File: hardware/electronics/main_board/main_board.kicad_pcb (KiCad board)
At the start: 2 copper layers, 5 parts

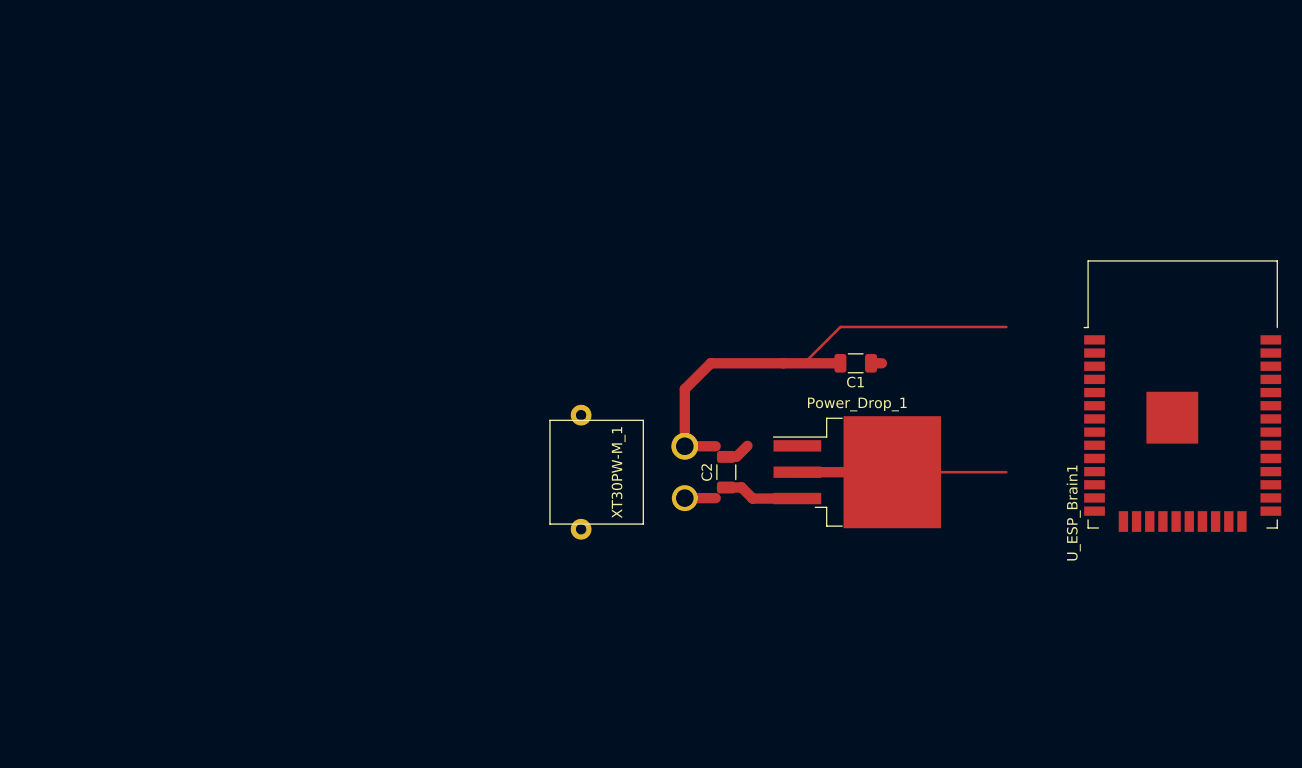
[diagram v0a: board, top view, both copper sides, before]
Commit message: pcb looking much better
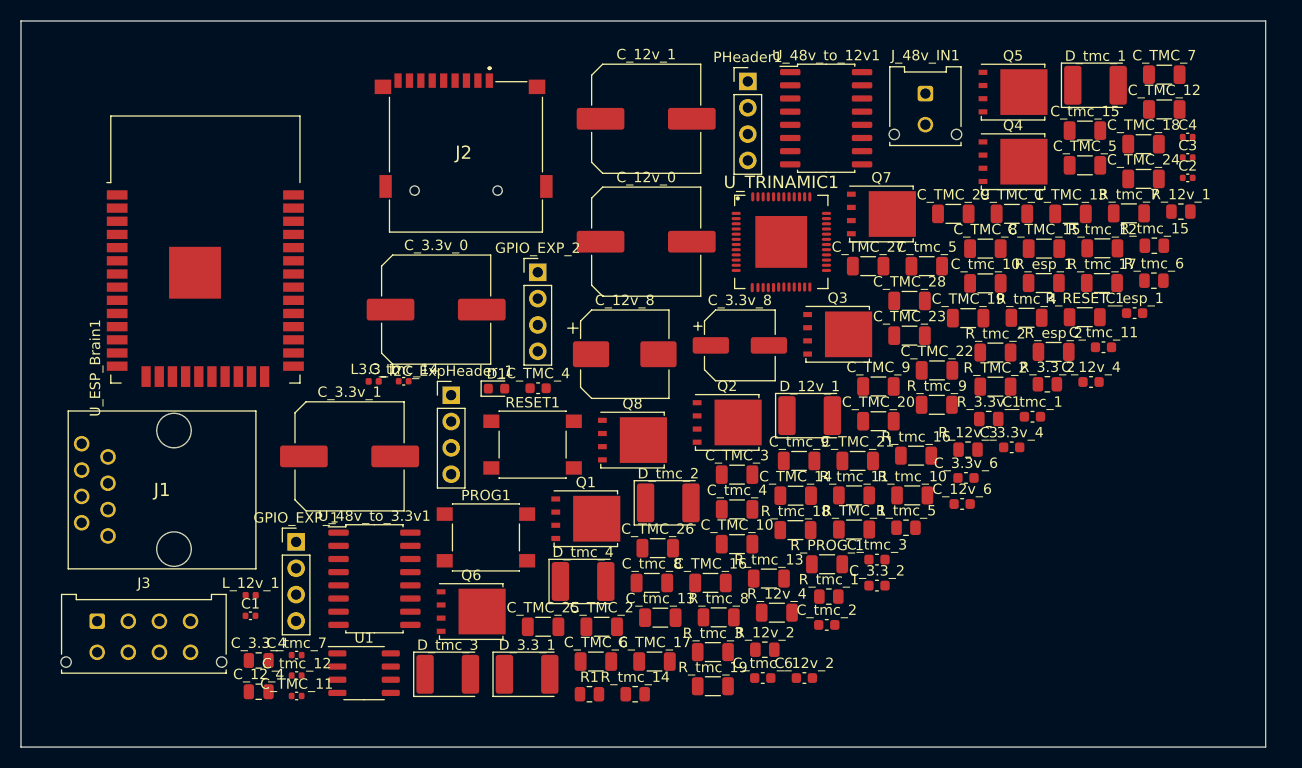
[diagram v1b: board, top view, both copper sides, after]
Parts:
- removed Power_Drop_1: LM1085-3.3, Package_TO_SOT_SMD:TO-263-3_TabPin2
- removed XT30PW-M_1: 24v DC In, main_board:XT30PW-M
- added C3: 10uF, Capacitor_SMD:C_0402_1005Metric, F.Cu at (172.5, 53.2)
- added C4: 100nF, Capacitor_SMD:C_0402_1005Metric, F.Cu at (172.5, 51.2)
- added C_12_4: 22nF, Capacitor_SMD:C_0805_2012Metric, F.Cu at (82.9, 104.7)
- added C_12v_0: 220uF, Capacitor_SMD:C_Elec_10x10.2, F.Cu at (120.3, 61.3)
- added C_12v_1: 220uF, Capacitor_SMD:C_Elec_10x10.2, F.Cu at (120.3, 49.4)
- added C_12v_2: 2.7nF, Capacitor_SMD:C_0603_1608Metric, F.Cu at (135.5, 103.3)
- added C_12v_4: 100nF, Capacitor_SMD:C_0603_1608Metric, F.Cu at (163.2, 74.8)
- added C_12v_6: 100nF, Capacitor_SMD:C_0603_1608Metric, F.Cu at (150.7, 86.6)
- added C_12v_8: 330uF, Capacitor_SMD:CP_Elec_8x10, F.Cu at (118.2, 72.1)
- added C_3.3_2: 2.7nF, Capacitor_SMD:C_0603_1608Metric, F.Cu at (142.5, 94.4)
- added C_3.3_4: 22nF, Capacitor_SMD:C_0805_2012Metric, F.Cu at (82.9, 101.7)
- added C_3.3v_0: 220uF, Capacitor_SMD:C_Elec_10x10.2, F.Cu at (100.0, 67.8)
- added C_3.3v_1: 220uF, Capacitor_SMD:C_Elec_10x10.2, F.Cu at (91.7, 82.0)
- added C_3.3v_4: 100nF, Capacitor_SMD:C_0603_1608Metric, F.Cu at (155.5, 81.1)
- added C_3.3v_6: 100nF, Capacitor_SMD:C_0603_1608Metric, F.Cu at (151.1, 84.1)
- added C_3.3v_8: 330uF, Capacitor_SMD:CP_Elec_6.3x5.9, F.Cu at (129.3, 71.3)
- added C_TMC_1: 1n, Capacitor_SMD:C_1206_3216Metric, F.Cu at (155.5, 58.6)
- added C_TMC_10: 1n, Capacitor_SMD:C_1206_3216Metric, F.Cu at (129.0, 90.4)
- added C_TMC_11: 100n, Capacitor_SMD:C_0402_1005Metric, F.Cu at (86.6, 105.1)
- added C_TMC_12: 1n, Capacitor_SMD:C_1206_3216Metric, F.Cu at (170.2, 48.5)
- added C_TMC_13: 1n, Capacitor_SMD:C_1206_3216Metric, F.Cu at (161.2, 58.6)
- added C_TMC_14: 100nF, Capacitor_SMD:C_1206_3216Metric, F.Cu at (134.7, 85.8)
- added C_TMC_15: 1n, Capacitor_SMD:C_1206_3216Metric, F.Cu at (158.6, 61.9)
- added C_TMC_16: 1n, Capacitor_SMD:C_1206_3216Metric, F.Cu at (126.5, 94.2)
- added C_TMC_17: 1n, Capacitor_SMD:C_1206_3216Metric, F.Cu at (121.1, 101.8)
- added C_TMC_18: 1n, Capacitor_SMD:C_1206_3216Metric, F.Cu at (168.2, 51.9)
- added C_TMC_19: 1n, Capacitor_SMD:C_1206_3216Metric, F.Cu at (151.3, 68.6)
- added C_TMC_2: 1n, Capacitor_SMD:C_1206_3216Metric, F.Cu at (116.0, 98.4)
- added C_TMC_20: 1n, Capacitor_SMD:C_1206_3216Metric, F.Cu at (142.7, 78.6)
- added C_TMC_21: 1n, Capacitor_SMD:C_1206_3216Metric, F.Cu at (140.7, 82.4)
- added C_TMC_22: 1n, Capacitor_SMD:C_1206_3216Metric, F.Cu at (148.3, 73.7)
- added C_TMC_23: 1n, Capacitor_SMD:C_1206_3216Metric, F.Cu at (145.7, 70.3)
- added C_TMC_24: 1n, Capacitor_SMD:C_1206_3216Metric, F.Cu at (168.2, 55.2)
- added C_TMC_25: 1n, Capacitor_SMD:C_1206_3216Metric, F.Cu at (110.3, 98.4)
- added C_TMC_26: 1n, Capacitor_SMD:C_1206_3216Metric, F.Cu at (121.4, 90.8)
- added C_TMC_27: 1n, Capacitor_SMD:C_1206_3216Metric, F.Cu at (141.7, 63.6)
- added C_TMC_28: 1n, Capacitor_SMD:C_1206_3216Metric, F.Cu at (145.7, 67.0)
- added C_TMC_29: 1n, Capacitor_SMD:C_1206_3216Metric, F.Cu at (149.9, 58.6)
- added C_TMC_3: 1n, Capacitor_SMD:C_1206_3216Metric, F.Cu at (129.0, 83.7)
- added C_TMC_4: 100nF, Capacitor_SMD:C_0603_1608Metric, F.Cu at (109.9, 75.4)
- added C_TMC_5: 1n, Capacitor_SMD:C_1206_3216Metric, F.Cu at (162.6, 53.9)
- added C_TMC_6: 1n, Capacitor_SMD:C_1206_3216Metric, F.Cu at (115.4, 101.8)
- added C_TMC_7: 1n, Capacitor_SMD:C_1206_3216Metric, F.Cu at (170.2, 45.2)
- added C_TMC_8: 1n, Capacitor_SMD:C_1206_3216Metric, F.Cu at (153.0, 61.9)
- added C_TMC_9: 1n, Capacitor_SMD:C_1206_3216Metric, F.Cu at (142.7, 75.2)
- added C_esp_1: 470n, Capacitor_SMD:C_0603_1608Metric, F.Cu at (167.4, 68.2)
- added C_tmc_1: 2.2u, Capacitor_SMD:C_0603_1608Metric, F.Cu at (157.5, 78.2)
- added C_tmc_10: 220nF, Capacitor_SMD:C_1206_3216Metric, F.Cu at (153.0, 65.3)
- added C_tmc_11: 2.2u, Capacitor_SMD:C_0603_1608Metric, F.Cu at (164.4, 71.5)
- added C_tmc_12: 100nF, Capacitor_SMD:C_0402_1005Metric, F.Cu at (86.6, 103.1)
- added C_tmc_13: 4.7uF, Capacitor_SMD:C_1206_3216Metric, F.Cu at (121.6, 97.5)
- added C_tmc_14: 100nF, Capacitor_SMD:C_0402_1005Metric, F.Cu at (96.9, 74.7)
- added C_tmc_15: 4.7uF, Capacitor_SMD:C_1206_3216Metric, F.Cu at (162.6, 50.6)
- added C_tmc_2: 2.2u, Capacitor_SMD:C_0603_1608Metric, F.Cu at (137.7, 98.2)
- added C_tmc_3: 470n, Capacitor_SMD:C_0603_1608Metric, F.Cu at (142.5, 91.9)
- added C_tmc_4: 220nF, Capacitor_SMD:C_1206_3216Metric, F.Cu at (129.0, 87.1)
- added C_tmc_5: 220nF, Capacitor_SMD:C_1206_3216Metric, F.Cu at (147.3, 63.6)
- added C_tmc_6: 2.2u, Capacitor_SMD:C_0603_1608Metric, F.Cu at (131.5, 103.3)
- added C_tmc_7: 100nF, Capacitor_SMD:C_0402_1005Metric, F.Cu at (86.6, 101.1)
- added C_tmc_8: 470nF, Capacitor_SMD:C_1206_3216Metric, F.Cu at (120.8, 94.2)
- added C_tmc_9: 220nF, Capacitor_SMD:C_1206_3216Metric, F.Cu at (135.0, 82.4)
- added D1: LED, LED_SMD:LED_0603_1608Metric, F.Cu at (105.8, 75.4)
- added D_12v_1: STPS3L60U, Diode_SMD:D_2114_3652Metric, F.Cu at (136.0, 78.0)
- added D_3.3_1: STPS3L60U, Diode_SMD:D_2114_3652Metric, F.Cu at (108.8, 103.0)
- added D_tmc_1: STPS3L60U, Diode_SMD:D_2114_3652Metric, F.Cu at (163.6, 46.2)
- added D_tmc_2: STPS3L60U, Diode_SMD:D_2114_3652Metric, F.Cu at (122.4, 86.5)
- added D_tmc_3: STPS3L60U, Diode_SMD:D_2114_3652Metric, F.Cu at (101.1, 103.0)
- added D_tmc_4: STPS3L60U, Diode_SMD:D_2114_3652Metric, F.Cu at (114.2, 94.0)
- added GPIO_EXP_1: Conn_01x04_Male, Connector_PinHeader_2.54mm:PinHeader_1x04_P2.54mm_Vertical, F.Cu at (86.5, 90.2)
- added GPIO_EXP_2: Conn_01x04_Male, Connector_PinHeader_2.54mm:PinHeader_1x04_P2.54mm_Vertical, F.Cu at (109.8, 64.2)
- added I2C_ExpHeader_1: Conn_01x04_Male, Connector_PinHeader_2.54mm:PinHeader_1x04_P2.54mm_Vertical, F.Cu at (101.5, 76.1)
- added J1: 215877-1, main_board:2158771, F.Cu at (65.9, 80.8)
- added J2: TF-15X15, main_board:TF15X15, F.Cu at (102.7, 52.7)
- added J3: Conn_02x04_Odd_Even, Connector_Molex:Molex_Micro-Fit_3.0_43045-0812_2x04_P3.00mm_Vertical, F.Cu at (67.3, 97.9)
- added J_48v_IN1: Molex, Connector_Molex:Molex_Micro-Fit_3.0_43045-0212_2x01_P3.00mm_Vertical, F.Cu at (147.2, 47.0)
- added L3.3_1: 126uH, Inductor_SMD:L_0402_1005Metric, F.Cu at (94.0, 74.7)
- added L_12v_1: 126uH, Inductor_SMD:L_0402_1005Metric, F.Cu at (82.1, 95.4)
- added PHeader1: Conn_01x04_Male, Connector_PinHeader_2.54mm:PinHeader_1x04_P2.54mm_Vertical, F.Cu at (130.1, 45.8)
- added PROG1: SW_Push_Dual_x2, Button_Switch_SMD:SW_Push_1P1T_NO_6x6mm_H9.5mm, F.Cu at (104.8, 89.8)
- added Q1: CSD18537NQ5A, Package_TO_SOT_SMD:TDSON-8-1, F.Cu at (114.5, 88.0)
- added Q2: CSD18537NQ5A, Package_TO_SOT_SMD:TDSON-8-1, F.Cu at (128.1, 78.7)
- added Q3: CSD18537NQ5A, Package_TO_SOT_SMD:TDSON-8-1, F.Cu at (138.7, 70.2)
- added Q4: CSD18537NQ5A, Package_TO_SOT_SMD:TDSON-8-1, F.Cu at (155.6, 53.6)
- added Q5: CSD18537NQ5A, Package_TO_SOT_SMD:TDSON-8-1, F.Cu at (155.6, 46.9)
- added Q6: CSD18537NQ5A, Package_TO_SOT_SMD:TDSON-8-1, F.Cu at (103.4, 96.9)
- added Q7: CSD18537NQ5A, Package_TO_SOT_SMD:TDSON-8-1, F.Cu at (143.0, 58.6)
- added Q8: CSD18537NQ5A, Package_TO_SOT_SMD:TDSON-8-1, F.Cu at (119.0, 80.4)
- added R1: 300 Ohms, Resistor_SMD:R_0805_2012Metric, F.Cu at (114.8, 104.9)
- added RESET1: SW_Push_Dual_x2, Button_Switch_SMD:SW_Push_1P1T_NO_6x6mm_H9.5mm, F.Cu at (109.3, 80.8)
- added R_12v_1: 20Kohms, Resistor_SMD:R_0805_2012Metric, F.Cu at (171.8, 58.4)
- added R_12v_2: 9.1kohms, Resistor_SMD:R_0805_2012Metric, F.Cu at (131.7, 100.6)
- added R_12v_3: 12kOhms, Resistor_SMD:R_0805_2012Metric, F.Cu at (151.3, 81.3)
- added R_12v_4: 4.7KOhms, Resistor_SMD:R_1206_3216Metric, F.Cu at (132.9, 97.0)
- added R_3.3_2: 9.1kohms, Resistor_SMD:R_0805_2012Metric, F.Cu at (159.0, 75.0)
- added R_3.3v_1: 20Kohms, Resistor_SMD:R_0805_2012Metric, F.Cu at (153.3, 78.4)
- added R_PROG_1: 10kOhms, Resistor_SMD:R_1206_3216Metric, F.Cu at (137.7, 92.4)
- added R_RESET_1: 10kOhms, Resistor_SMD:R_1206_3216Metric, F.Cu at (162.6, 68.6)
- added R_TMC_1: 10kOhms, Resistor_SMD:R_1206_3216Metric, F.Cu at (140.3, 89.0)
- added R_TMC_2: 10kOhms, Resistor_SMD:R_1206_3216Metric, F.Cu at (153.9, 75.3)
- added R_esp_1: 4.7KOhms, Resistor_SMD:R_1206_3216Metric, F.Cu at (158.6, 65.3)
- added R_esp_2: 4.7KOhms, Resistor_SMD:R_1206_3216Metric, F.Cu at (159.6, 71.9)
- added R_tmc_1: 2R2, Resistor_SMD:R_0805_2012Metric, F.Cu at (137.9, 95.5)
- added R_tmc_10: 10Ohm, Resistor_SMD:R_1206_3216Metric, F.Cu at (145.9, 85.7)
- added R_tmc_11: 10Ohm, Resistor_SMD:R_1206_3216Metric, F.Cu at (140.3, 85.7)
- added R_tmc_12: 10Ohm, Resistor_SMD:R_1206_3216Metric, F.Cu at (164.3, 61.9)
- added R_tmc_13: 10Ohm, Resistor_SMD:R_1206_3216Metric, F.Cu at (132.1, 93.8)
- added R_tmc_14: 47R, Resistor_SMD:R_0805_2012Metric, F.Cu at (119.2, 104.9)
- added R_tmc_15: 47R, Resistor_SMD:R_0805_2012Metric, F.Cu at (169.3, 61.7)
- added R_tmc_16: 10Ohm, Resistor_SMD:R_1206_3216Metric, F.Cu at (146.3, 81.9)
- added R_tmc_17: 10Ohm, Resistor_SMD:R_1206_3216Metric, F.Cu at (164.2, 65.3)
- added R_tmc_18: 10Ohm, Resistor_SMD:R_1206_3216Metric, F.Cu at (134.7, 89.1)
- added R_tmc_19: 10Ohm, Resistor_SMD:R_1206_3216Metric, F.Cu at (126.7, 104.1)
- added R_tmc_2: 10Ohm, Resistor_SMD:R_1206_3216Metric, F.Cu at (153.9, 72.0)
- added R_tmc_3: 10Ohm, Resistor_SMD:R_1206_3216Metric, F.Cu at (126.7, 100.8)
- added R_tmc_4: 10Ohm, Resistor_SMD:R_1206_3216Metric, F.Cu at (156.9, 68.6)
- added R_tmc_5: 47R, Resistor_SMD:R_0805_2012Metric, F.Cu at (145.3, 88.9)
- added R_tmc_6: 47R, Resistor_SMD:R_0805_2012Metric, F.Cu at (169.2, 65.0)
- added R_tmc_7: 10Ohm, Resistor_SMD:R_1206_3216Metric, F.Cu at (166.8, 58.5)
- added R_tmc_8: 10Ohm, Resistor_SMD:R_1206_3216Metric, F.Cu at (127.3, 97.5)
- added R_tmc_9: 10Ohm, Resistor_SMD:R_1206_3216Metric, F.Cu at (148.3, 77.0)
- added U1: P82B96, Package_SO:SO-8_3.9x4.9mm_P1.27mm, F.Cu at (93.1, 102.9)
- added U_48v_to_12v1: L4978D, Package_SO:SO-16_5.3x10.2mm_P1.27mm, F.Cu at (137.6, 49.4)
- added U_48v_to_3.3v1: L4978D, Package_SO:SO-16_5.3x10.2mm_P1.27mm, F.Cu at (94.1, 93.8)
- added U_TRINAMIC1: TMC5160-TA, trinamic-footprints:eTQFP48, F.Cu at (133.3, 61.3)
- C1: footprint Capacitor_SMD:C_1206_3216Metric -> Capacitor_SMD:C_0402_1005Metric
- C2: value 10uF -> 100nF; footprint Capacitor_SMD:C_1206_3216Metric -> Capacitor_SMD:C_0402_1005Metric
- moved U_ESP_Brain1 95.3 mm to (77.8, 65.0)
- moved C1 63.2 mm to (82.1, 97.3), turned to 0 degrees
- moved C2 52.8 mm to (172.5, 55.1), turned to 0 degrees
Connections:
- C1 pad 1: +3V3 -> 3.3v_Program
- C1 pad 2: Earth -> 3.3v_Program
- C2 pad 1: +24V -> 3.3v_Program
- C2 pad 2: Earth -> 3.3v_Program
- U_ESP_Brain1 pad 1: Net-(U_ESP_Brain1-Pad1) -> 3.3v_Program
- U_ESP_Brain1 pad 10: (no net) -> ESP_GPIO_25
- U_ESP_Brain1 pad 11: (no net) -> ESP_GPIO_26
- U_ESP_Brain1 pad 12: (no net) -> ESP_GPIO_27
- U_ESP_Brain1 pad 13: (no net) -> HSPI_CLK
- U_ESP_Brain1 pad 14: (no net) -> HSPI_MISO
- U_ESP_Brain1 pad 15: Net-(U_ESP_Brain1-Pad1) -> 3.3v_Program
- U_ESP_Brain1 pad 16: (no net) -> HSPI_MOSI
- U_ESP_Brain1 pad 17: (no net) -> Net-(U_ESP_Brain1-Pad17)
- U_ESP_Brain1 pad 18: (no net) -> Net-(U_ESP_Brain1-Pad18)
- U_ESP_Brain1 pad 19: (no net) -> Net-(U_ESP_Brain1-Pad19)
- U_ESP_Brain1 pad 2: (no net) -> 3.3v_Program
- U_ESP_Brain1 pad 20: (no net) -> Net-(U_ESP_Brain1-Pad20)
- U_ESP_Brain1 pad 21: (no net) -> Net-(U_ESP_Brain1-Pad21)
- U_ESP_Brain1 pad 22: (no net) -> Net-(U_ESP_Brain1-Pad22)
- U_ESP_Brain1 pad 23: (no net) -> HSPI_CS
- U_ESP_Brain1 pad 24: (no net) -> ESP_LED
- U_ESP_Brain1 pad 25: (no net) -> Program
- U_ESP_Brain1 pad 26: (no net) -> ESP_GPIO_4
- U_ESP_Brain1 pad 27: (no net) -> ESP_GPIO_16
- U_ESP_Brain1 pad 28: (no net) -> ESP_GPIO_17
- U_ESP_Brain1 pad 29: (no net) -> VSPI_CS
- U_ESP_Brain1 pad 3: (no net) -> Reset
- U_ESP_Brain1 pad 30: (no net) -> VSPI_CLK
- U_ESP_Brain1 pad 31: (no net) -> VSPI_MISO
- U_ESP_Brain1 pad 32: (no net) -> Net-(U_ESP_Brain1-Pad32)
- U_ESP_Brain1 pad 33: (no net) -> ESP_I2C_SDA
- U_ESP_Brain1 pad 34: (no net) -> RX_Program
- U_ESP_Brain1 pad 35: (no net) -> TX_Program
- U_ESP_Brain1 pad 36: (no net) -> ESP_I2C_SCL
- U_ESP_Brain1 pad 37: (no net) -> VSPI_MOSI
- U_ESP_Brain1 pad 38: Net-(U_ESP_Brain1-Pad1) -> 3.3v_Program
- U_ESP_Brain1 pad 39: Net-(U_ESP_Brain1-Pad1) -> 3.3v_Program
- U_ESP_Brain1 pad 4: (no net) -> Net-(U_ESP_Brain1-Pad4)
- U_ESP_Brain1 pad 5: (no net) -> ESP_Emergency
- U_ESP_Brain1 pad 6: (no net) -> Net-(U_ESP_Brain1-Pad6)
- U_ESP_Brain1 pad 7: (no net) -> Net-(U_ESP_Brain1-Pad7)
- U_ESP_Brain1 pad 8: (no net) -> ESP_GPIO_32
- U_ESP_Brain1 pad 9: (no net) -> ESP_GPIO_33
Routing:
- net Earth: track 49.0 -> 0.00 mm
- net +3V3: track 21.2 -> 0.00 mm
- net +24V: track 10.3 -> 0.00 mm
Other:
- board outline added: 120 x 70 mm
